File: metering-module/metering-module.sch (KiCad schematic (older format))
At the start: 38 parts, among them J1 North, J2 South, J3 West, J4 East, Q1 MMBT3904, Q2 MMBT3904, U1 LTV-817S, U2 LTV-817S, U3 BA033CC0FP-E2, U4 MAX3486, U5 MAX3486

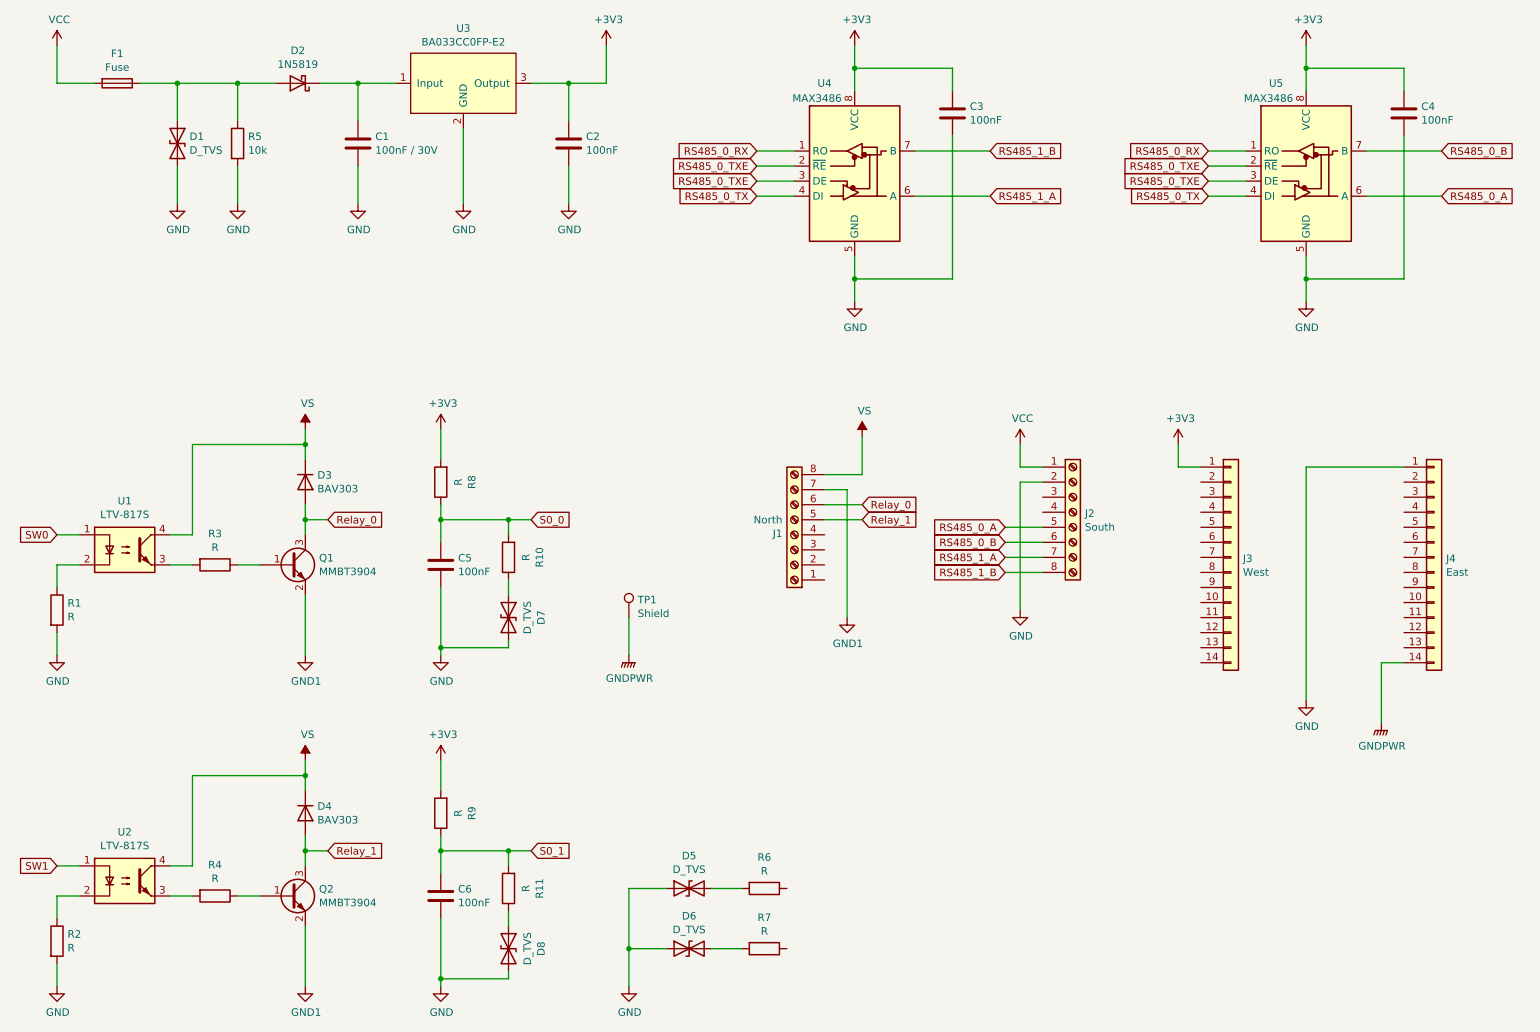
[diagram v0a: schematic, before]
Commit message: Ongoing Work. Still not ready for small and dedicated commits.
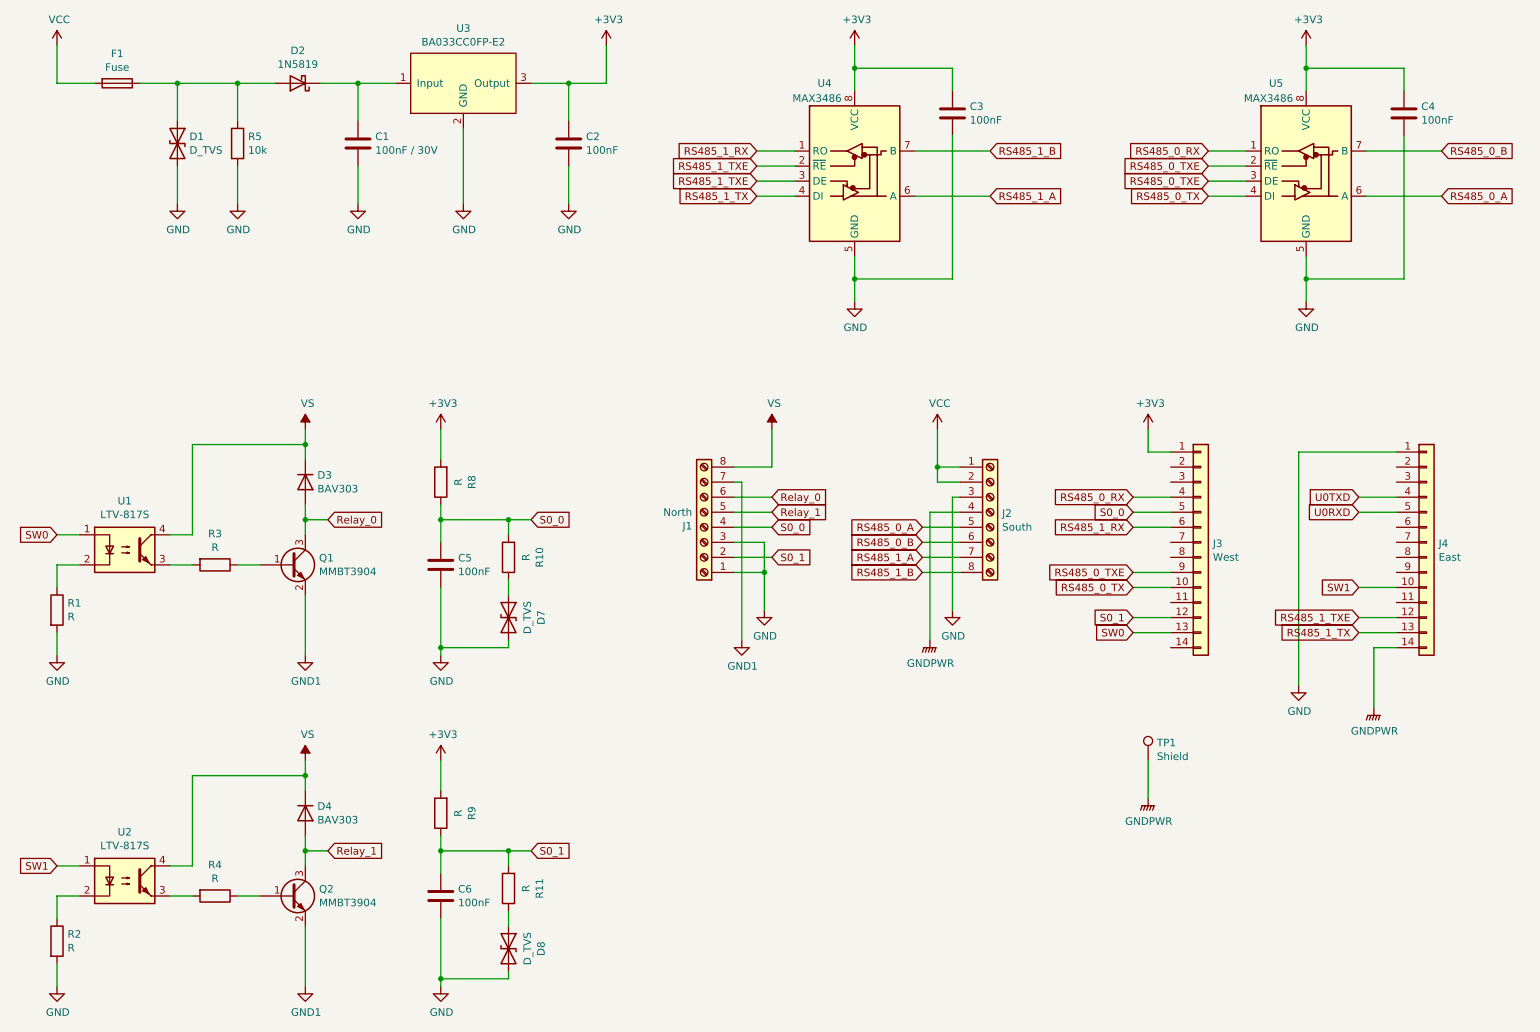
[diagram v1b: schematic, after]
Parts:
- removed D5, D6: D_TVS, Diode_SMD:D_0603_1608Metric_Pad1.05x0.95mm_HandSolder, symbol Device:D_TVS
- removed R6, R7: R, Resistor_SMD:R_1206_3216Metric_Pad1.30x1.75mm_HandSolder, symbol Device:R
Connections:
- net GND: now also J1.1 (Pin_1), J1.3 (Pin_3), J2.3 (Pin_3); no longer J2.2 (Pin_2)
- net GNDPWR: now also J2.4 (Pin_4)
- net RS485_0_RX: now also J3.4 (Pin_4); no longer U4.1 (RO)
- net RS485_0_TX: now also J3.10 (Pin_10); no longer U4.4 (DI)
- net RS485_0_TXE: now also J3.9 (Pin_9); no longer U4.2 (~RE), U4.3 (DE)
- net S0_0: now also J1.4 (Pin_4), J3.5 (Pin_5)
- net S0_1: now also J1.2 (Pin_2), J3.12 (Pin_12)
- net SW0: now also J3.13 (Pin_13)
- net SW1: now also J4.10 (Pin_10)
- net VCC: now also J2.2 (Pin_2)
- net RS485_1_RX: now reaches J3.6 (Pin_6)
- net RS485_1_RX: now also U4.1 (RO)
- net RS485_1_TXE: now reaches J4.12 (Pin_12)
- net RS485_1_TXE: now also U4.2 (~RE), U4.3 (DE)
- net RS485_1_TX: now reaches J4.13 (Pin_13)
- net RS485_1_TX: now also U4.4 (DI)
- net U0TXD: now reaches J4.4 (Pin_4)
- net U0RXD: now reaches J4.5 (Pin_5)
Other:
- moved on the sheet: J1, J2, J3, J4, TP1
